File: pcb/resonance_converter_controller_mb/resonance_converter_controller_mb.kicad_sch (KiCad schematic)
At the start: 36 parts, among them J3 Conn_01x02, Q1 Q_NPN_BEC, Q2 Q_NPN_BEC, Q3 Q_PMOS_GDS, U1 PCF8574RGTR, U2 TL431D, U3 74LVC1G04

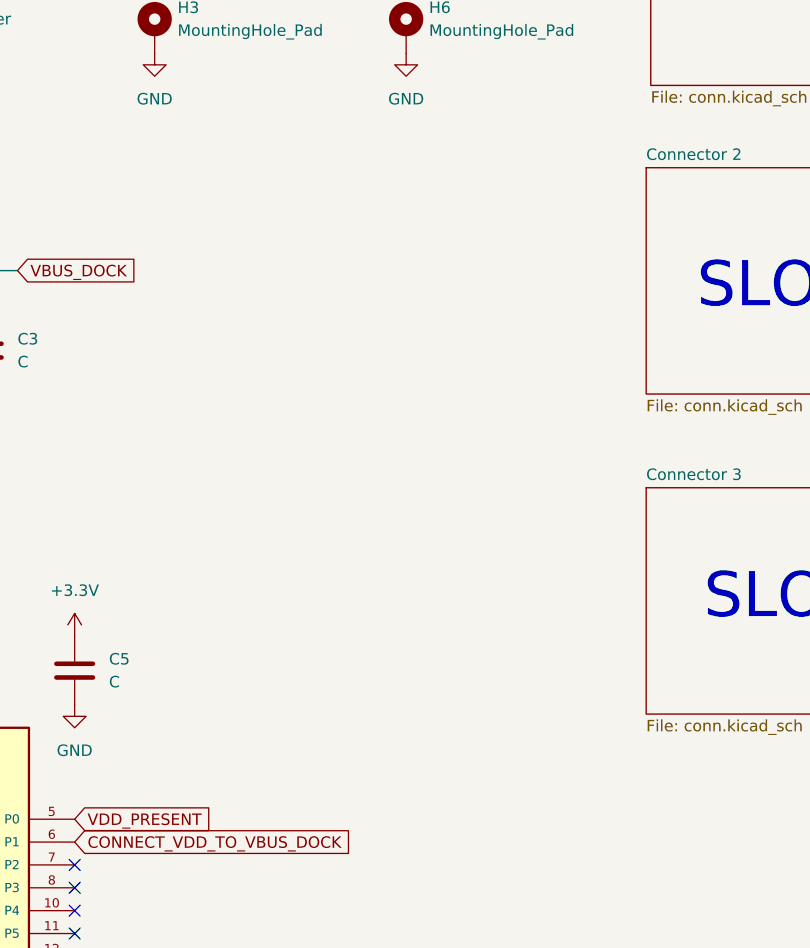
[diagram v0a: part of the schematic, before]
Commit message: _mb board freerouted
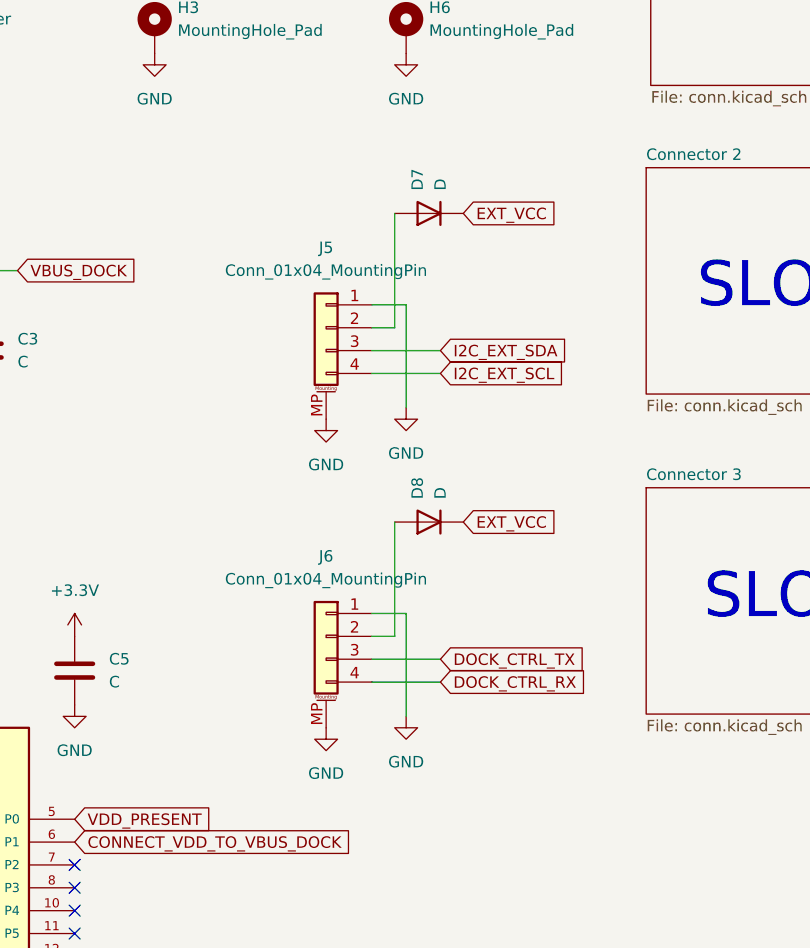
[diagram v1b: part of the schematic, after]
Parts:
- added D7, D8: D, Diode_SMD:D_SMA, symbol Device:D
- added J5, J6: Conn_01x04_MountingPin, Connector_JST:JST_SH_SM04B-SRSS-TB_1x04-1MP_P1.00mm_Horizontal, symbol Connector_Generic_MountingPin:Conn_01x04_MountingPin
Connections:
- net EXT_VCC: now also D7.1 (K), D8.1 (K)
- net GND: now also J5.1 (Pin_1), J5.MP (MountPin), J6.1 (Pin_1), J6.MP (MountPin)
- net I2C_EXT_SCL: now also J5.4 (Pin_4)
- net I2C_EXT_SDA: now also J5.3 (Pin_3)
- new net: D8.2 (A), J6.2 (Pin_2)
- new net: D7.2 (A), J5.2 (Pin_2)
- new net DOCK_CTRL_RX: J6.4 (Pin_4)
- new net DOCK_CTRL_TX: J6.3 (Pin_3)
